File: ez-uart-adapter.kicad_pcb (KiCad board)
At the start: 2 copper layers, 45 x 15 mm, 25 parts, among them J1 USB_C_Receptacle_USB2.0_16P, J2 Conn_01x04_Pin, Q1 2N7002, Q2 2N7002, Q3 AO3401A, SW1 MK-11C04-G013, U1 USBLC6-2SC6, U2 AP2112K-3.3, U3 CH340C

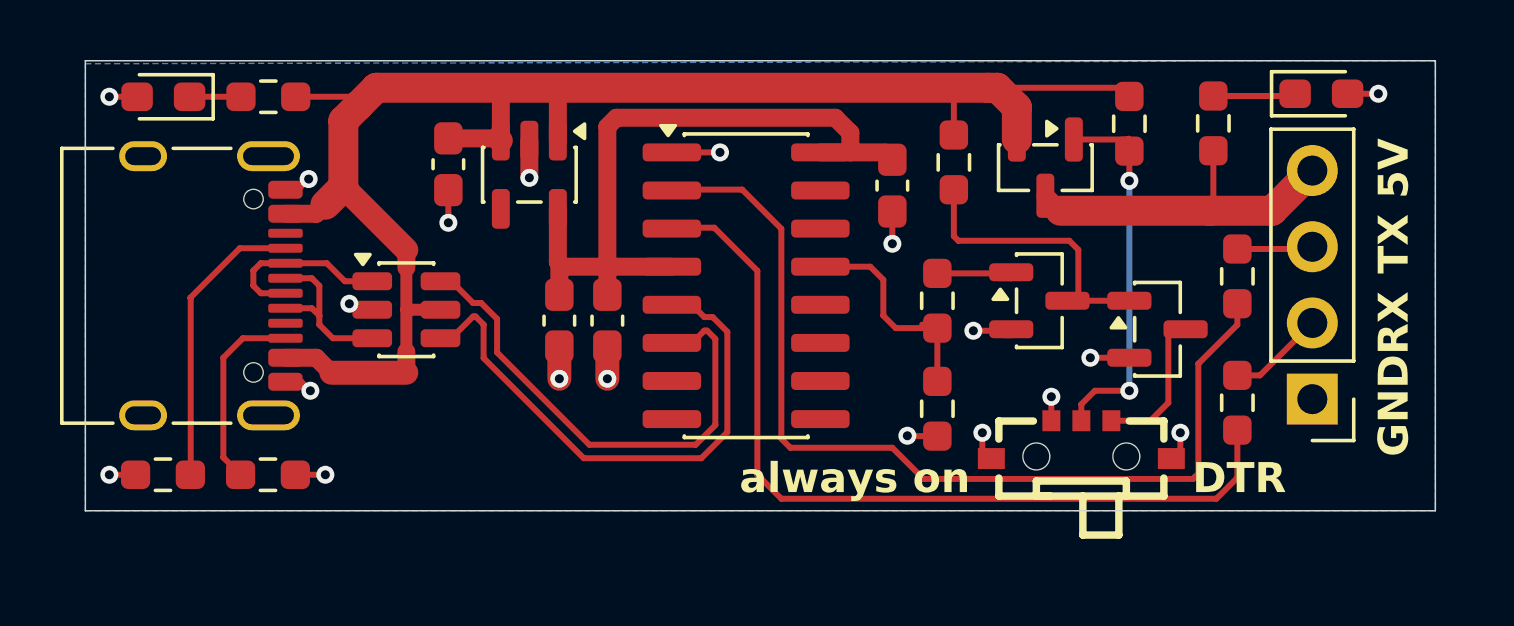
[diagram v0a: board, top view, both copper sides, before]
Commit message: fixup! Add ESD protection to UART
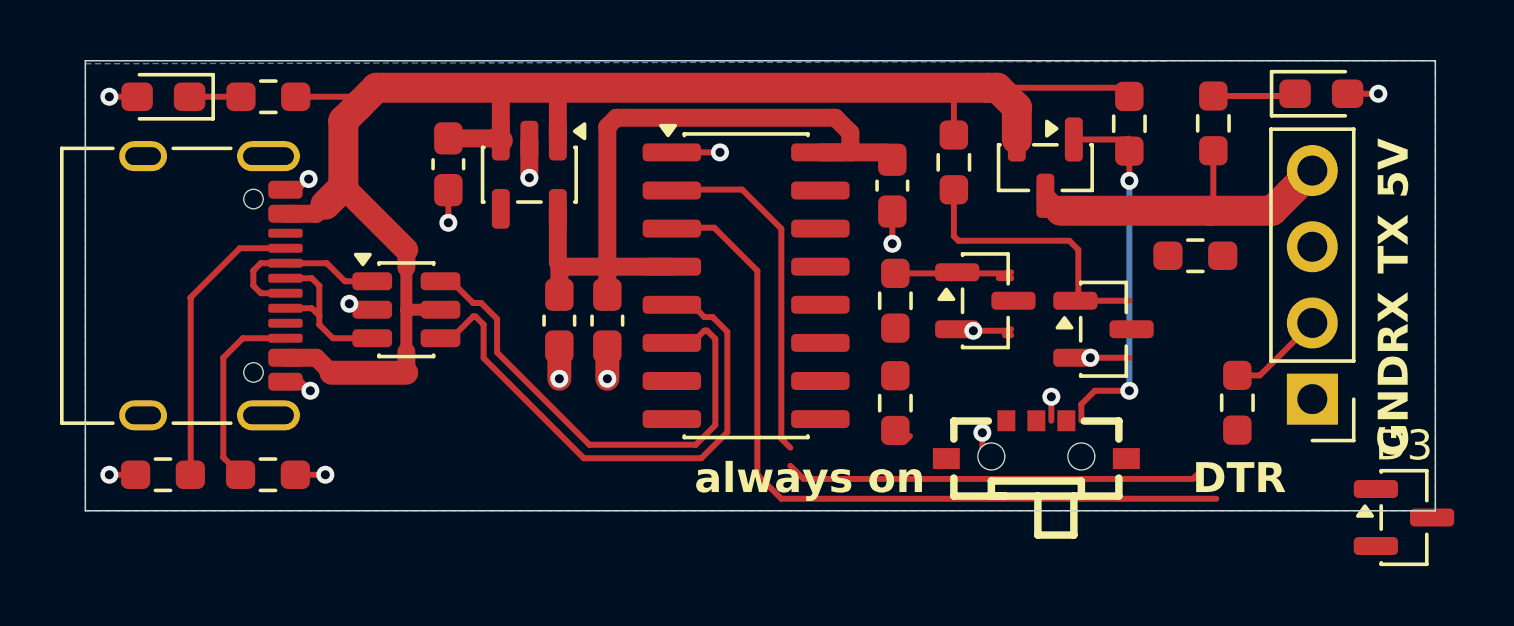
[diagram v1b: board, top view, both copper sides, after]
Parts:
- added D3: PSM712, Package_TO_SOT_SMD:SOT-23, F.Cu at (170.0, 112.7)
- moved Q1 1.80 mm to (156.0, 105.5)
- moved Q2 1.80 mm to (159.9, 106.5)
- moved R9 1.56 mm to (163.0, 104.0), turned to 180 degrees
- moved SW1 1.50 mm to (157.7, 110.1)
- moved R7 1.41 mm to (153.0, 108.9)
- moved R6 1.40 mm to (153.0, 105.5)
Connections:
- D1 pad 1: Net-(D1-K) -> GND
- D1 pad 2: GND -> Net-(D1-A)
- D2 pad 1: Net-(D2-K) -> GND
- D2 pad 2: GND -> Net-(D2-A)
- R1 pad 2: Net-(D1-K) -> Net-(D1-A)
- R8 pad 2: Net-(D2-K) -> Net-(D2-A)
- R9 pad 1: TX -> Net-(J2-Pin_3)
- R9 pad 2: Net-(J2-Pin_3) -> TX
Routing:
- net TX: track 32.0 -> 11.7 mm
- net Net-(J2-Pin_3): track 2.81 -> 14.2 mm
- net Net-(U3-~{DTR}): track 7.90 -> 0.01 mm
- net Net-(Q2-D): track 5.69 -> 0.00 mm
- net RX: track 28.6 -> 26.0 mm
- net Net-(D2-K): track 2.56 -> 0.00 mm
- net Net-(D1-K): track 2.00 -> 0.00 mm
- net Net-(Q1-G): track 3.12 -> 4.52 mm
- net Net-(D2-A): track 0.00 -> 1.03 mm
- net Net-(D1-A): track 0.00 -> 0.92 mm
- net GND: track 19.3 -> 20.0 mm, vias 19 -> 17
